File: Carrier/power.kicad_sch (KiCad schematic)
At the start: 49 parts, among them J8 USB_C_Receptacle_USB2.0_16P, Q1 AO3400A, Q3 AO3400A, U10 EL817S1C, U12 USBLC6-2SC6, U2 IP5306, U9 EL817S1C

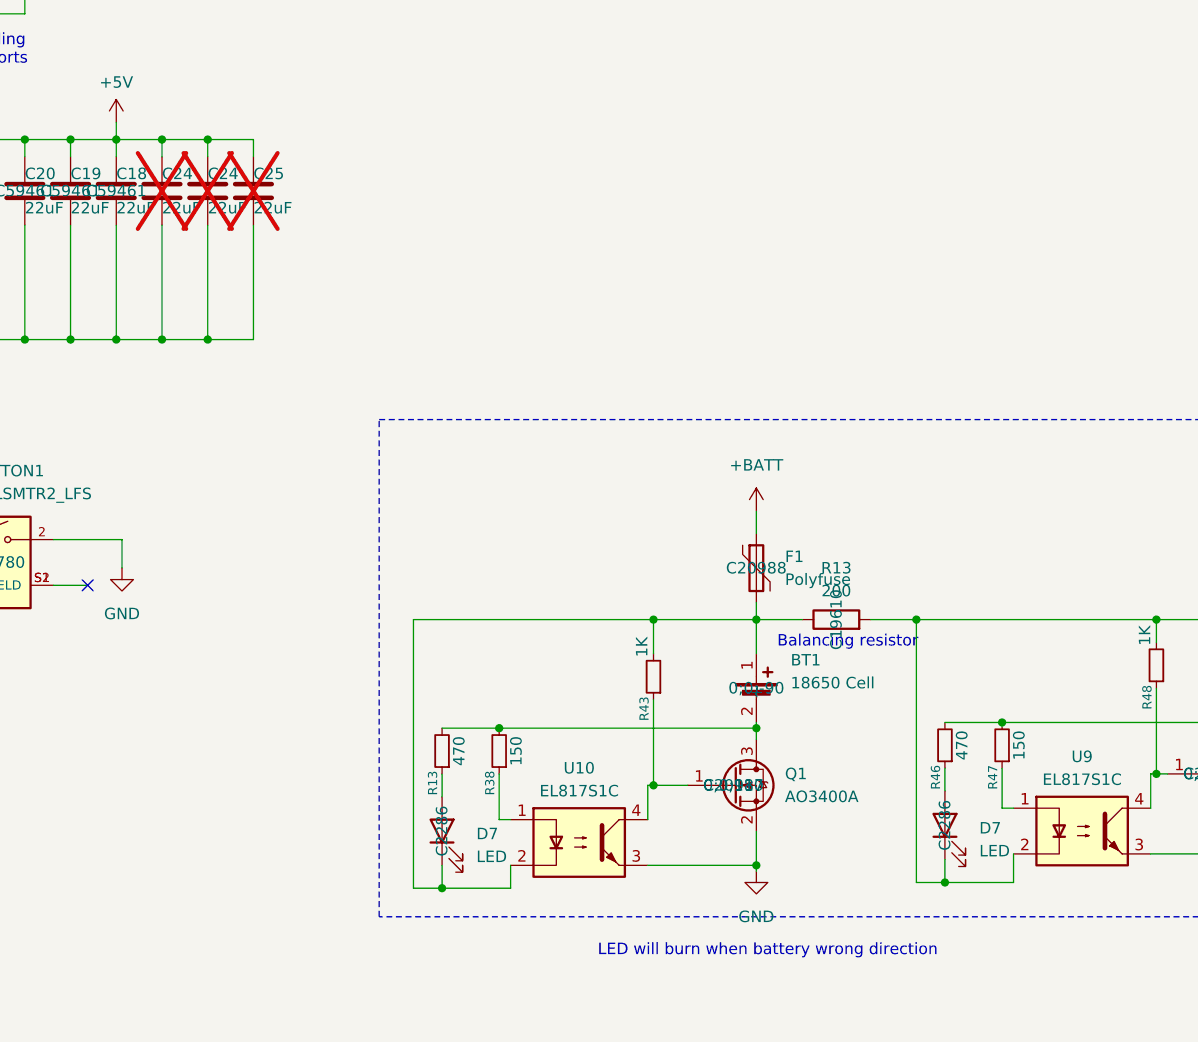
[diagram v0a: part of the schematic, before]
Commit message: fix annotation
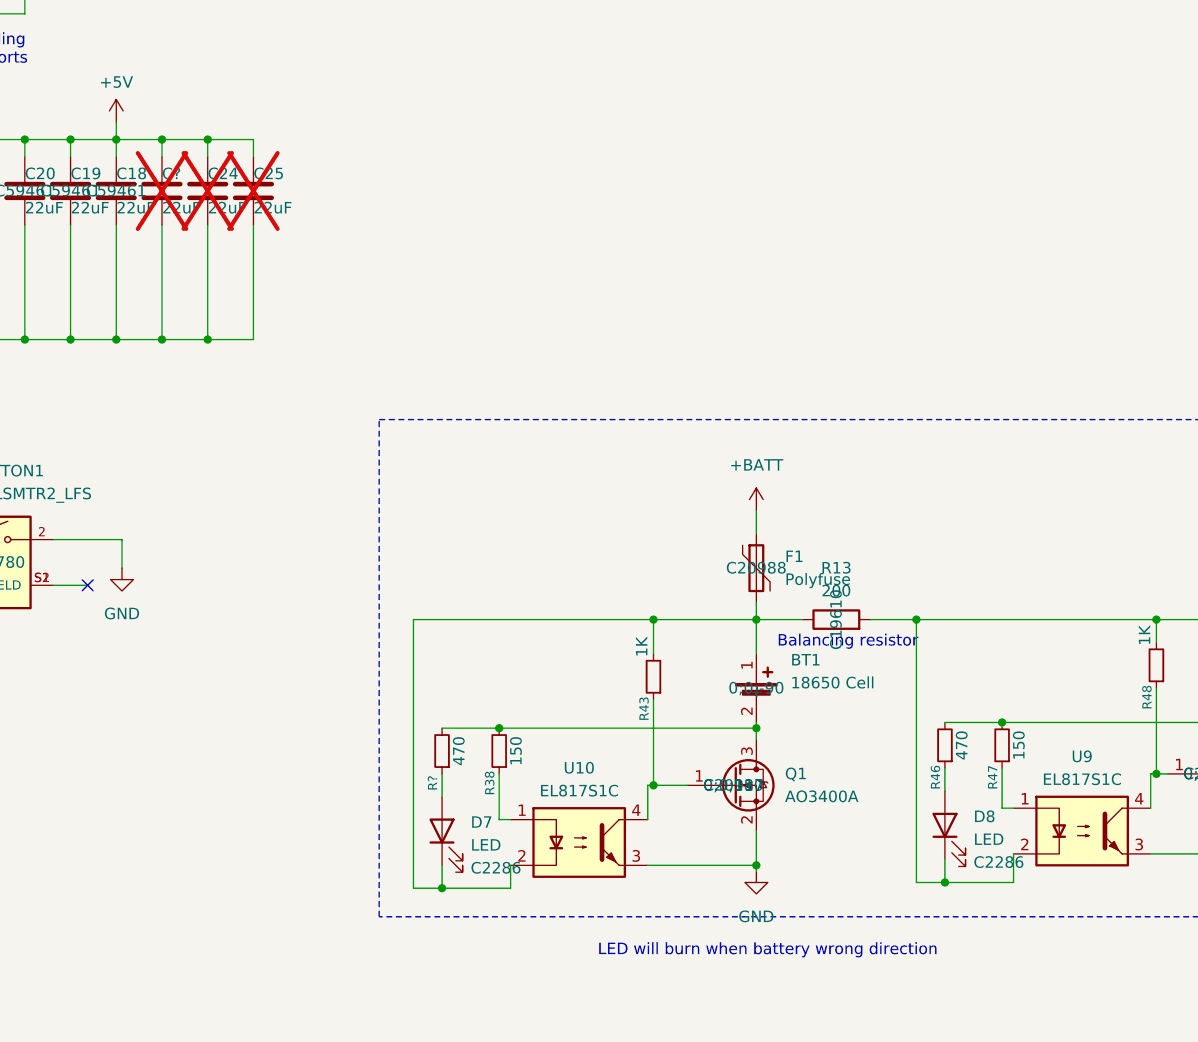
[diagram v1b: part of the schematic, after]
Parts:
- renumbered C24 to C?, D7 to D8, R13 to R?
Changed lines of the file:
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@@
 		(dnp no)
 		(fields_autoplaced yes)
-		(property "Reference" "D7"
-			(at 234.315 137.4774 90)
+		(property "Reference" "D8"
+			(at 233.68 136.2074 90)
 			(effects
 				(font
@@
 		)
 		(property "Value" "LED"
-			(at 234.315 140.0174 90)
+			(at 233.68 138.7474 90)
 			(effects
 				(font
@@
 		)
 		(property "LCSC" "C2286"
-			(at 230.505 137.16 0)
+			(at 233.68 141.2874 90)
 			(effects
 				(font
 					(size 1.27 1.27)
 				)
+				(justify right)
 			)
 		)
@@
 			(project "badgeCarrierCard"
 				(path "/d0a98fce-b133-4503-8f8a-83b2a1eed591/05158df8-c1e6-40b8-af8c-4aba99cbc568"
-					(reference "D7")
+					(reference "D8")
 					(unit 1)
 				)
@@
 		(fields_autoplaced yes)
 		(property "Reference" "D7"
-			(at 178.435 138.1124 90)
+			(at 177.8 136.8424 90)
 			(effects
 				(font
@@
 		)
 		(property "Value" "LED"
-			(at 178.435 140.6524 90)
+			(at 177.8 139.3824 90)
 			(effects
 				(font
@@
 		)
 		(property "LCSC" "C2286"
-			(at 174.625 137.795 0)
+			(at 177.8 141.9224 90)
 			(effects
 				(font
 					(size 1.27 1.27)
 				)
+				(justify right)
 			)
 		)
@@
 		(on_board yes)
 		(dnp no)
-		(property "Reference" "R13"
+		(property "Reference" "R?"
 			(at 173.609 132.461 90)
 			(effects
@@
 			(project "badgeCarrierCard"
 				(path "/d0a98fce-b133-4503-8f8a-83b2a1eed591/05158df8-c1e6-40b8-af8c-4aba99cbc568"
-					(reference "R13")
+					(reference "R?")
 					(unit 1)
 				)
@@
 		(on_board yes)
 		(dnp yes)
-		(property "Reference" "C24"
+		(property "Reference" "C?"
 			(at 143.51 64.77 0)
 			(effects
@@
 			(project "badgeCarrierCard"
 				(path "/d0a98fce-b133-4503-8f8a-83b2a1eed591/05158df8-c1e6-40b8-af8c-4aba99cbc568"
-					(reference "C24")
+					(reference "C?")
 					(unit 1)
 				)
